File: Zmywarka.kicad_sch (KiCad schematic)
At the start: 66 parts, among them J1 Conn_01x08, Q1 BC817, Q2 BC817, Q3 BC817, Q4 BC817, SW1 SW_Omron_B3FS, SW2 SW_Omron_B3FS, SW3 SW_Omron_B3FS, SW4 SW_Omron_B3FS, U1 74HC595, U2 74HC595

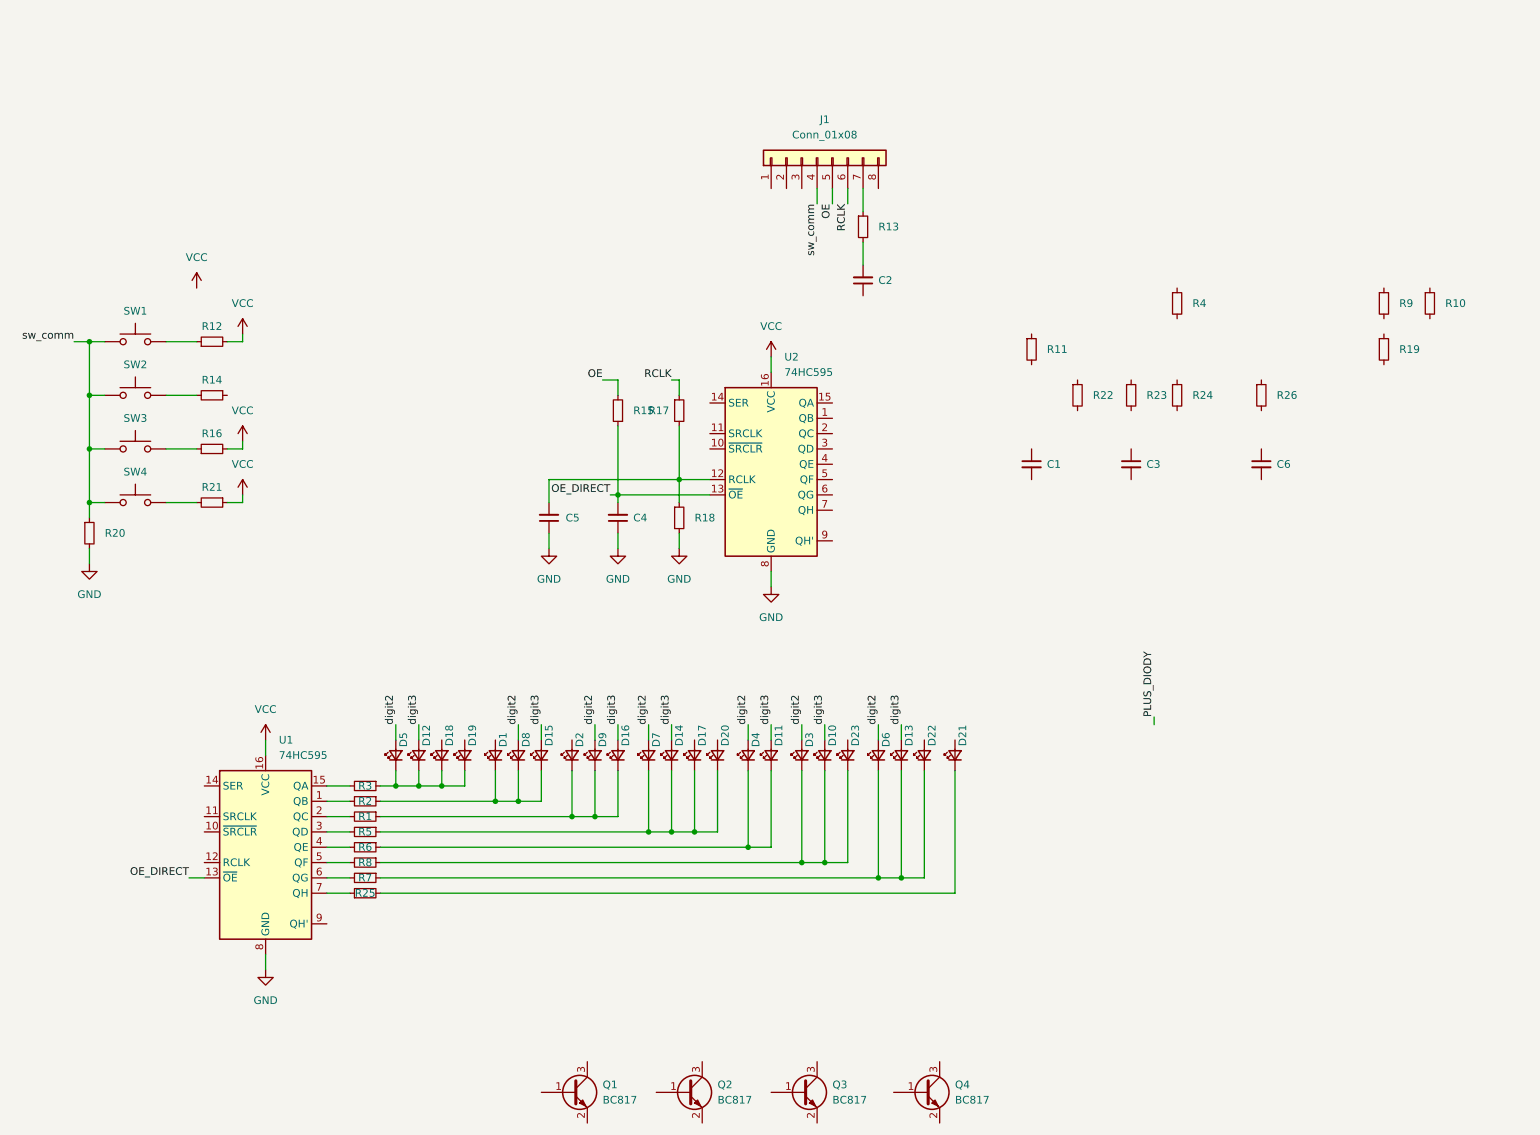
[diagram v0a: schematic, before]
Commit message: almost done
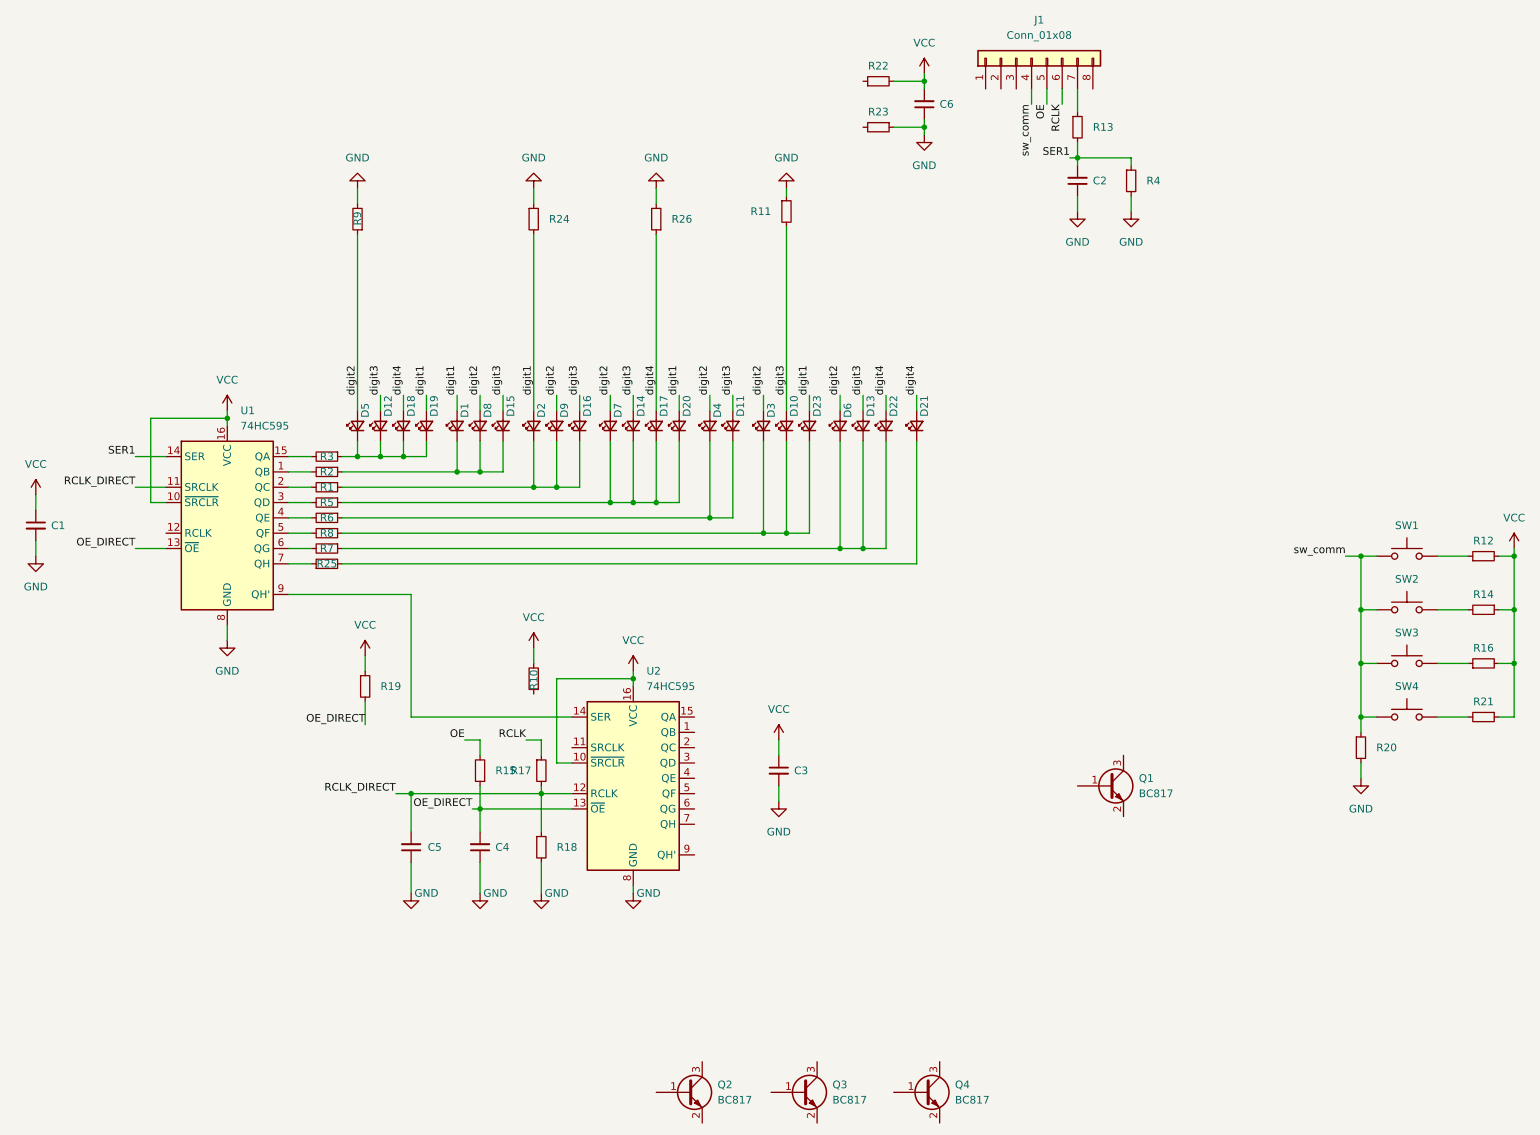
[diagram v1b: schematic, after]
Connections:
- net GND: now also C1.2, C2.1, C3.2, C6.1, R11.1, R23.1, R24.1, R26.2, R4.2, R9.2
- net OE_DIRECT: now also R19.2
- net VCC: now also C1.1, C3.1, C6.2, R10.2, R14.1, R19.1, R22.2, U1.10 (~{SRCLR}), U2.10 (~{SRCLR})
- net digit2: now also R9.1
- net digit3: now also R11.2
- net RCLK_DIRECT: now reaches C5.2, R17.2, R18.1, U2.12 (RCLK)
- net RCLK_DIRECT: now also U1.11 (SRCLK)
- net at U2.14 (SER): now also U1.9 (QH')
- net SER1: now reaches R4.1
- net SER1: now also C2.2, R13.2, U1.14 (SER)
- net digit1: now reaches D20.2 (A)
- net digit1: now also D1.2 (A), D19.2 (A), D2.2 (A), D23.2 (A), R24.2
- net digit4: now reaches D21.2 (A)
- net digit4: now also D17.2 (A), D18.2 (A), D22.2 (A), R26.1
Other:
- moved on the sheet: C1, C2, C3, C4, C5, C6, D1, D10, D11, D12, D13, D14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
